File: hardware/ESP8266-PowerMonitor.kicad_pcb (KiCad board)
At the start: 2 copper layers, 31 x 41.1 mm, 9 parts, among them P1 CONN_LEFT, P2 CONN_RIGHT, P3 CONN_METER, P4 CONN_PIR, P5 CONN_POWER, P6 CONN_1WIRE

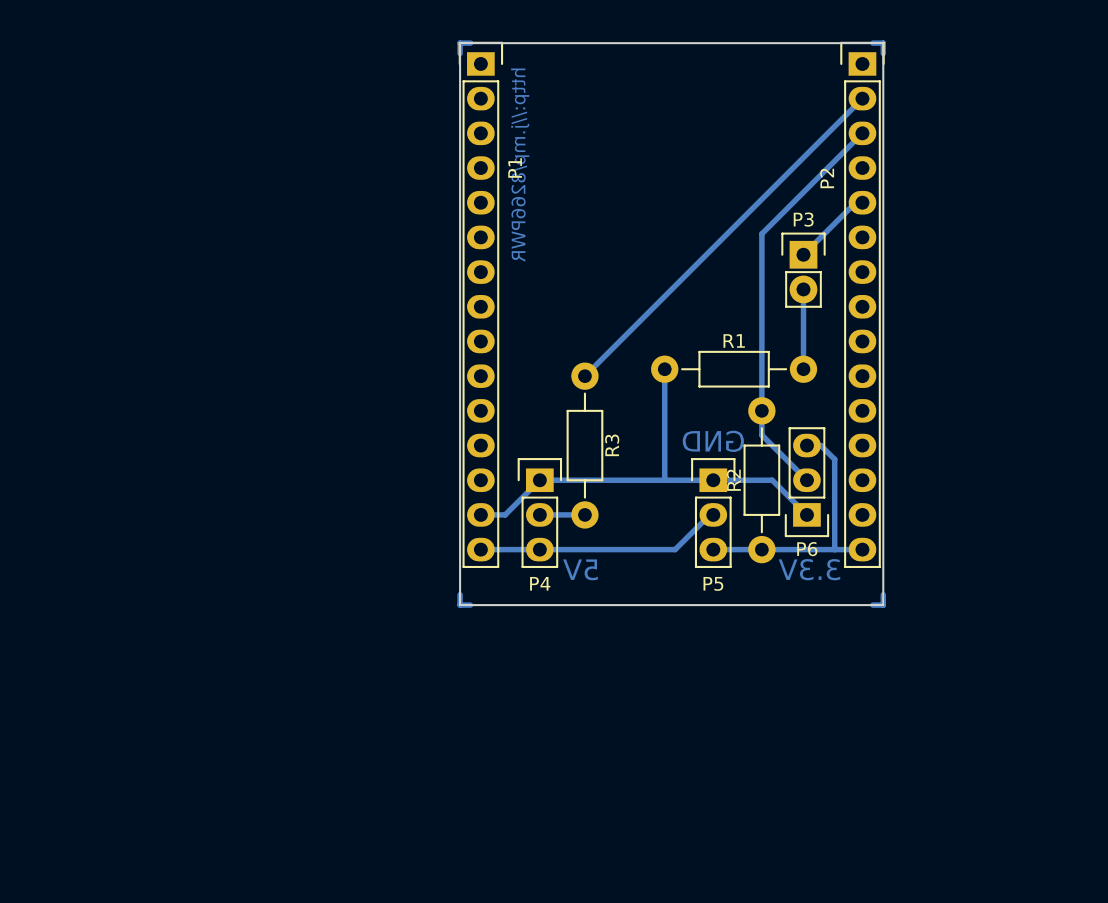
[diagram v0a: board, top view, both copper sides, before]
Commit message: Redesigned the board.
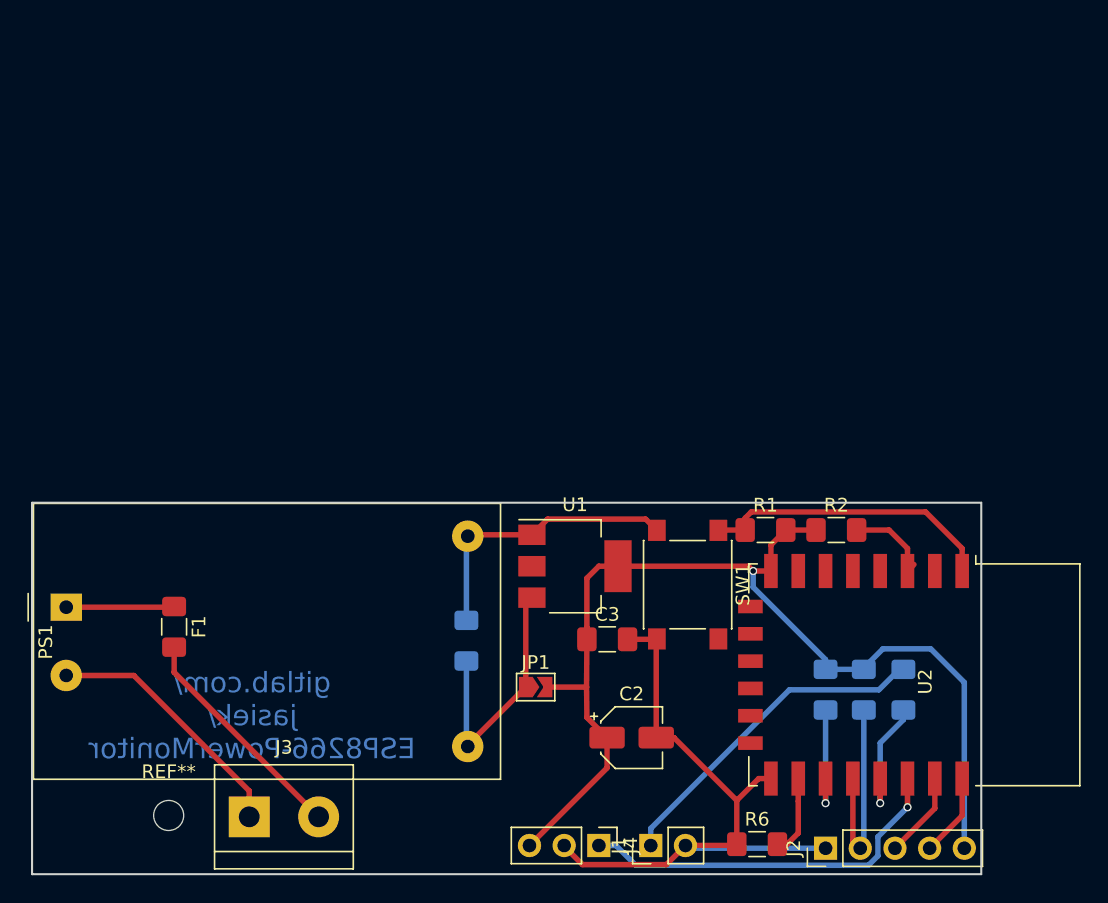
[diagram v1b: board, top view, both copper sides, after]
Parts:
- removed P1: CONN_LEFT, Socket_Strips:Socket_Strip_Straight_1x15
- removed P2: CONN_RIGHT, Socket_Strips:Socket_Strip_Straight_1x15
- removed P3: CONN_METER, Pin_Headers:Pin_Header_Straight_1x02
- removed P4: CONN_PIR, Pin_Headers:Pin_Header_Straight_1x03
- removed P5: CONN_POWER, Pin_Headers:Pin_Header_Straight_1x03
- removed P6: CONN_1WIRE, Pin_Headers:Pin_Header_Straight_1x03
- added C1: 0.1uF, Capacitor_SMD:C_1206_3216Metric_Pad1.42x1.75mm_HandSolder, B.Cu at (139.4, 100.9)
- added C2: 10uF, Capacitor_SMD:CP_Elec_4x5.3, F.Cu at (151.5, 108.0)
- added C3: 100nF, Capacitor_SMD:C_1206_3216Metric_Pad1.42x1.75mm_HandSolder, F.Cu at (149.7, 100.8)
- added F1: 100mA, Fuse:Fuse_1206_3216Metric_Pad1.42x1.75mm_HandSolder, F.Cu at (118.0, 99.9)
- added J1: CONN_PULSE, Connector_PinHeader_2.54mm:PinHeader_1x02_P2.54mm_Vertical, F.Cu at (152.9, 115.9)
- added J2: CONN_PROG, Connector_PinHeader_2.54mm:PinHeader_1x05_P2.54mm_Vertical, F.Cu at (165.7, 116.1)
- added J3: CONN_AC, TerminalBlock:TerminalBlock_bornier-2_P5.08mm, F.Cu at (123.5, 113.8)
- added J4: CONN_TEMP, Connector_PinHeader_2.54mm:PinHeader_1x03_P2.54mm_Vertical, F.Cu at (149.1, 115.9)
- added JP1: 3.3V BYPASS, Jumper:SolderJumper-2_P1.3mm_Open_TrianglePad1.0x1.5mm, F.Cu at (144.5, 104.3)
- added PS1: HLK-PM03, Converter_ACDC:Converter_ACDC_HiLink_HLK-PMxx, F.Cu at (110.1, 98.5)
- added R4: 10k, Resistor_SMD:R_1206_3216Metric_Pad1.42x1.75mm_HandSolder, B.Cu at (168.5, 104.5)
- added R5: 10k, Resistor_SMD:R_1206_3216Metric_Pad1.42x1.75mm_HandSolder, B.Cu at (165.7, 104.5)
- added R6: 10k, Resistor_SMD:R_1206_3216Metric_Pad1.42x1.75mm_HandSolder, F.Cu at (160.7, 115.8)
- added REF**: , MountingHole:MountingHole_2.2mm_M2, F.Cu at (117.6, 113.7)
- added SW1: SW_RESET, Button_Switch_SMD:SW_Push_1P1T_NO_6x6mm_H9.5mm, F.Cu at (155.6, 96.8)
- added U1: AMS1117-3.3, Package_TO_SOT_SMD:SOT-223-3_TabPin2, F.Cu at (147.3, 95.5)
- added U2: ESP-12F, RF_Module:ESP-12E, F.Cu at (172.2, 103.4)
- R1: value 470 -> 10k; footprint Resistors_ThroughHole:Resistor_Horizontal_RM10mm -> Resistor_SMD:R_1206_3216Metric_Pad1.42x1.75mm_HandSolder
- R2: value 2.2k -> 10k; footprint Resistors_ThroughHole:Resistor_Horizontal_RM10mm -> Resistor_SMD:R_1206_3216Metric_Pad1.42x1.75mm_HandSolder
- R3: footprint Resistors_ThroughHole:Resistor_Horizontal_RM10mm -> Resistor_SMD:R_1206_3216Metric_Pad1.42x1.75mm_HandSolder; moved to B.Cu
- moved R3 29.4 mm to (171.4, 104.5)
- moved R1 12.0 mm to (161.3, 92.8), turned to 0 degrees
- moved R2 6.56 mm to (166.5, 92.8), turned to 0 degrees
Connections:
- R1 pad 2: GND -> +3.3V
- R2 pad 1: 3.3V -> +3.3V
- R2 pad 2: GPIO4 -> Net-(R2-Pad2)
- R3 pad 2: GPIO5 -> PULSE
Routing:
- net +3.3V: track 0.00 -> 78.6 mm, vias 0 -> 1
- net GND: track 34.1 -> 68.7 mm
- net GPIO4: track 30.3 -> 0.00 mm
- net GPIO5: track 28.7 -> 0.00 mm
- net DS18B20_DQ: track 0.00 -> 27.9 mm, vias 0 -> 1
- net PULSE: track 0.00 -> 24.6 mm
- net 3.3V: track 20.0 -> 0.00 mm
- net Net-(C1-Pad1): track 0.00 -> 19.2 mm
- net AC-N: track 0.00 -> 18.8 mm
- net 5V: track 18.4 -> 0.00 mm
- net AC-L: track 0.00 -> 16.8 mm
- net Net-(R1-Pad1): track 5.84 -> 21.7 mm
- net _PROG: track 0.00 -> 15.6 mm
- net Net-(R5-Pad2): track 0.00 -> 8.62 mm, vias 0 -> 1
- net Net-(F1-Pad1): track 0.00 -> 7.92 mm
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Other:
- board size 31 x 41.1 mm -> 69.5 x 27.2 mm
- board text added: "0,8"
- board text added: "0,9"
- board text added: "10"
- board text added: "12,6"
- board text added: "17,9"
- board text added: "26,65"
- board text added: "27,1"
- board text added: "27,15"
- board text added: "28,85"
- board text added: "3,45"
- board text added: "30,95"
- board text added: "35,2"
- board text added: "5,35"
- board text added: "63,05"
- board text added: "7,05"
- board text added: "7,35"
- board text added: "72,1"
- board text added: "8,4"
- board text added: "90"
- board text added: "A"
- board text added: "gitlab.com/ jasiek/ ESP8266-PowerMonitor"
- board text removed: "3.3V"
- board text removed: "5V"
- board text removed: "GND"
- board text removed: "http://j.mp/8266PWR"
